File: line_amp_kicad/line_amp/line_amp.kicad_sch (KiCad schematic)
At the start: 0 parts

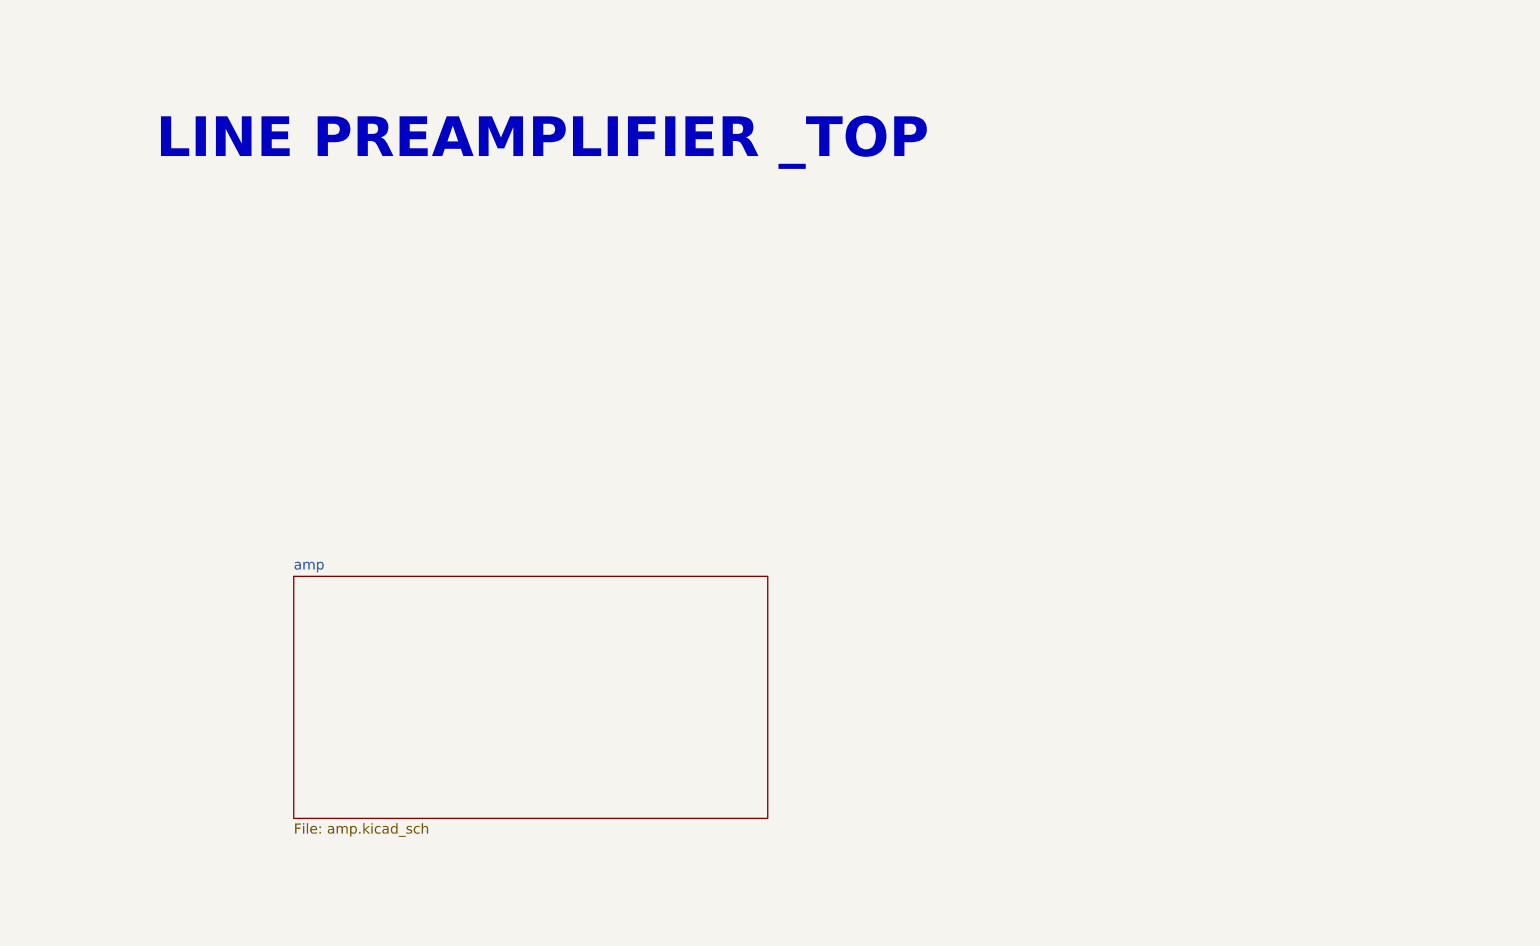
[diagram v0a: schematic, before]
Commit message: updates to schematics
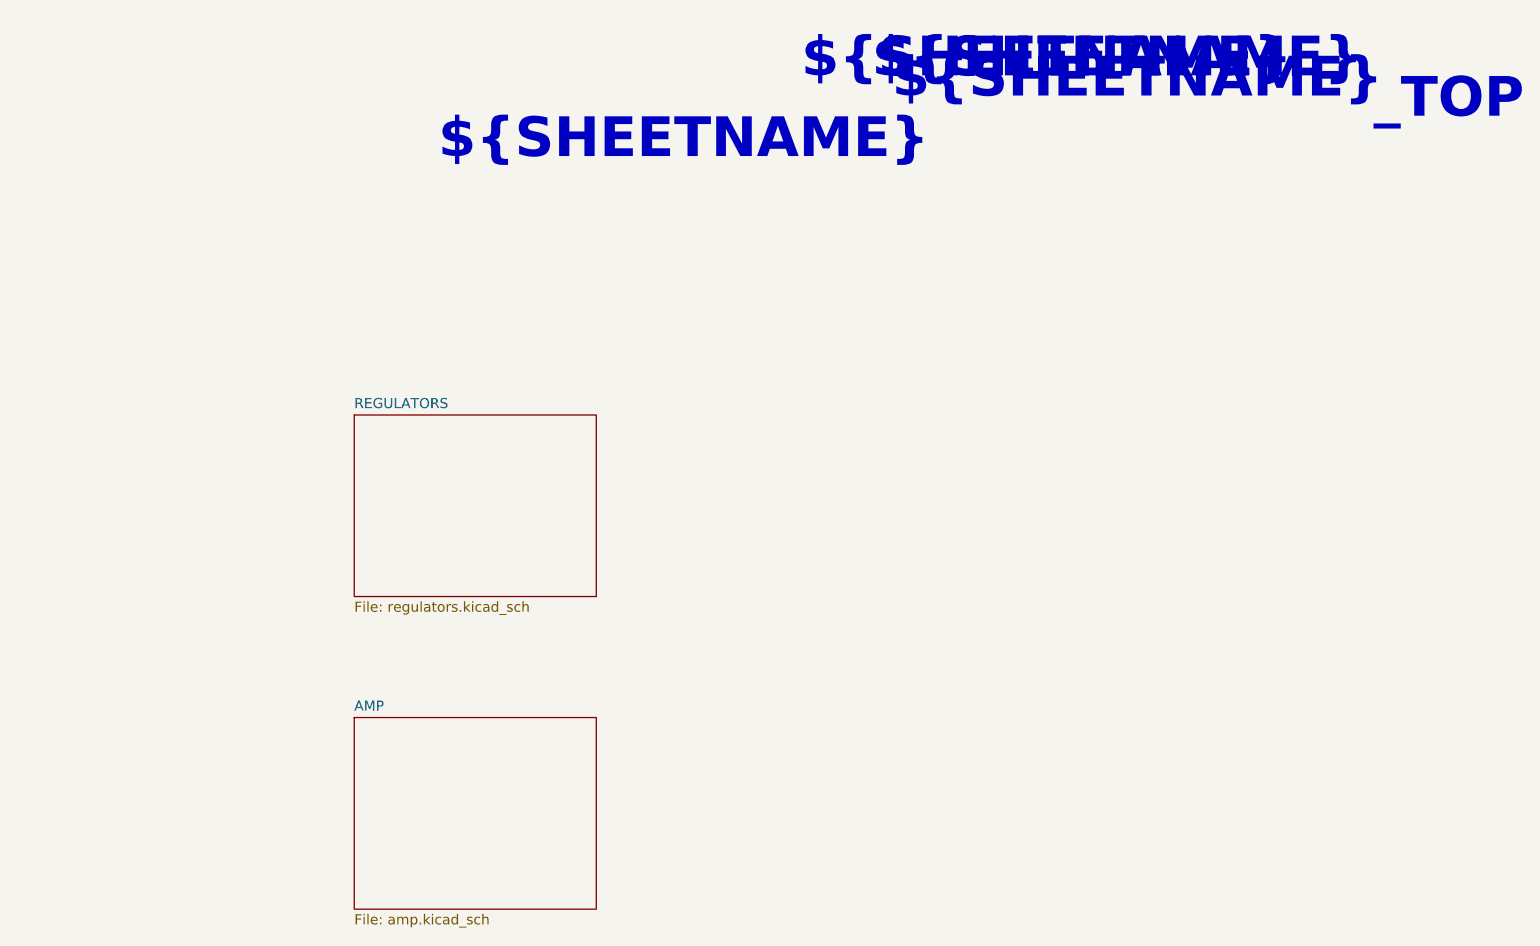
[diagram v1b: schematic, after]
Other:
- sheet amp renamed AMP
- added sheet REGULATORS (regulators.kicad_sch)
- note added: "${SHEETNAME}"
- note added: "_TOP"
- note removed: "LINE PREAMPLIFIER _TOP"
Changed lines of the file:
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@@
     (comment 6 "${PCBA_PROJ}")
   )
-  (text "LINE PREAMPLIFIER _TOP\n" (at 199.39 31.75 180)
+  (text "_TOP\n" (at 274.32 26.67 180)
     (effects (font (size 5 5) (thickness 1) bold) (justify right bottom))
   )
-  (sheet (at 119.38 83.82) (size 59.69 30.48) (fields_autoplaced)
+  (text "${SHEETNAME}\n" (at 245.11 21.59 180)
+    (effects (font (size 5 5) (thickness 1) bold) (justify right bottom))
+  )
+  (text "${SHEETNAME}\n" (at 254 21.59 180)
+    (effects (font (size 5 5) (thickness 1) bold) (justify right bottom))
+  )
+  (text "${SHEETNAME}" (at 199.39 31.75 180)
+    (effects (font (size 5 5) (thickness 1) bold) (justify right bottom))
+  )
+  (text "${SHEETNAME}\n" (at 256.54 24.13 180)
+    (effects (font (size 5 5) (thickness 1) bold) (justify right bottom))
+  )
+  (sheet (at 127 63.5) (size 30.48 22.86) (fields_autoplaced)
     (stroke (width 0.1524) (type solid) (color 0 0 0 0))
     (fill (color 0 0 0 0.0000))
-    (property "Sheet name" "amp" (id 0) (at 119.38 83.1084 0)
+    (property "Sheet name" "REGULATORS" (id 0) (at 127 62.7884 0)
       (effects (font (size 1.27 1.27)) (justify left bottom))
     )
-    (property "Sheet file" "amp.kicad_sch" (id 1) (at 119.38 114.8846 0)
+    (property "Sheet file" "regulators.kicad_sch" (id 1) (at 127 86.9446 0)
+      (effects (font (size 1.27 1.27)) (justify left top))
+    )
+  )
+  (sheet (at 127 101.6) (size 30.48 24.13) (fields_autoplaced)
+    (stroke (width 0.1524) (type solid) (color 0 0 0 0))
+    (fill (color 0 0 0 0.0000))
+    (property "Sheet name" "AMP" (id 0) (at 127 100.8884 0)
+      (effects (font (size 1.27 1.27)) (justify left bottom))
+    )
+    (property "Sheet file" "amp.kicad_sch" (id 1) (at 127 126.3146 0)
       (effects (font (size 1.27 1.27)) (justify left top))
     )
@@
     (path "/" (page "1"))
     (path "/86c9a117-d4e0-4b94-b683-c667aba115d1" (page "2"))
+    (path "/25f0dc4a-715b-4730-aa67-011162ff0e7d" (page "3"))
+  )
+  (symbol_instances
+    (path "/86c9a117-d4e0-4b94-b683-c667aba115d1/236282df-5239-4053-8372-dfc1e6f9323e"
+      (reference "#PWR?") (unit 1) (value "GND") (footprint "")
+    )
+    (path "/86c9a117-d4e0-4b94-b683-c667aba115d1/9485359b-1ec0-4221-bb01-0106d929b9f5"
+      (reference "R?") (unit 1) (value "1k") (footprint "")
+    )
+    (path "/86c9a117-d4e0-4b94-b683-c667aba115d1/ce25f997-29d0-47f3-a82a-57acc64259d8"
+      (reference "R?") (unit 1) (value "330") (footprint "")
+    )
+    (path "/86c9a117-d4e0-4b94-b683-c667aba115d1/571dd08f-0ed8-4e76-bf91-f5a224ee71ce"
+      (reference "U?") (unit 1) (value "LM4562") (footprint "")
+    )
+    (path "/86c9a117-d4e0-4b94-b683-c667aba115d1/98ba5dd3-97ee-447f-8351-875c0606d759"
+      (reference "U?") (unit 1) (value "LM4562") (footprint "")
+    )
+    (path "/86c9a117-d4e0-4b94-b683-c667aba115d1/456ef4ab-d417-4be2-99a2-df71bc1589a7"
+      (reference "U?") (unit 2) (value "LM4562") (footprint "")
+    )
+    (path "/86c9a117-d4e0-4b94-b683-c667aba115d1/8ba55066-02f2-4e5d-a63f-6f191fc4623d"
+      (reference "U?") (unit 2) (value "LM4562") (footprint "")
+    )
+    (path "/86c9a117-d4e0-4b94-b683-c667aba115d1/3318370f-2f86-41bf-bca4-3acd1719ba46"
+      (reference "U?") (unit 3) (value "LM4562") (footprint "")
+    )
+    (path "/86c9a117-d4e0-4b94-b683-c667aba115d1/3b375248-509e-4399-a63e-ea73287fefea"
+      (reference "U?") (unit 3) (value "LM4562") (footprint "")
+    )
   )
 )
